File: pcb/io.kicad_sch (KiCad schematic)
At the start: 31 parts, among them Q3 2N7002, Q4 2N7002, Q5 2N7002, Q6 2N7002, Q7 BT148, Q8 BT148

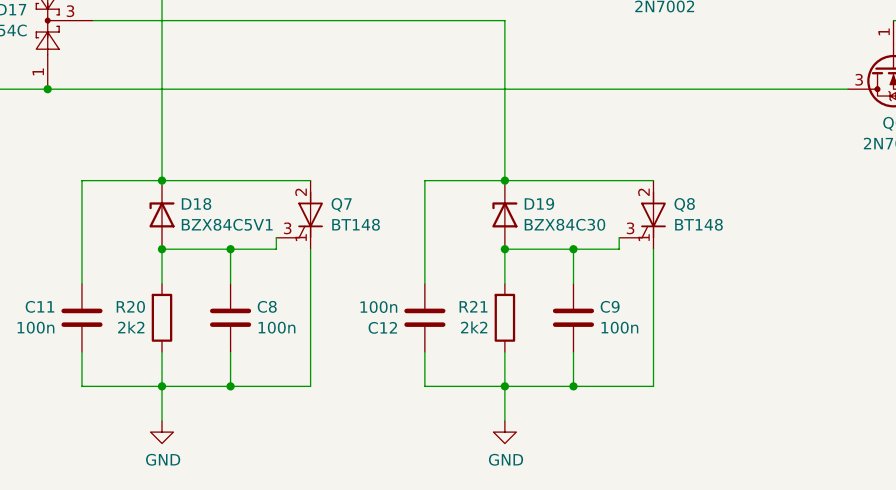
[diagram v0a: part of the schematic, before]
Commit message: Add protection on internal inputs, divide stepdown voltage measuring by 2.
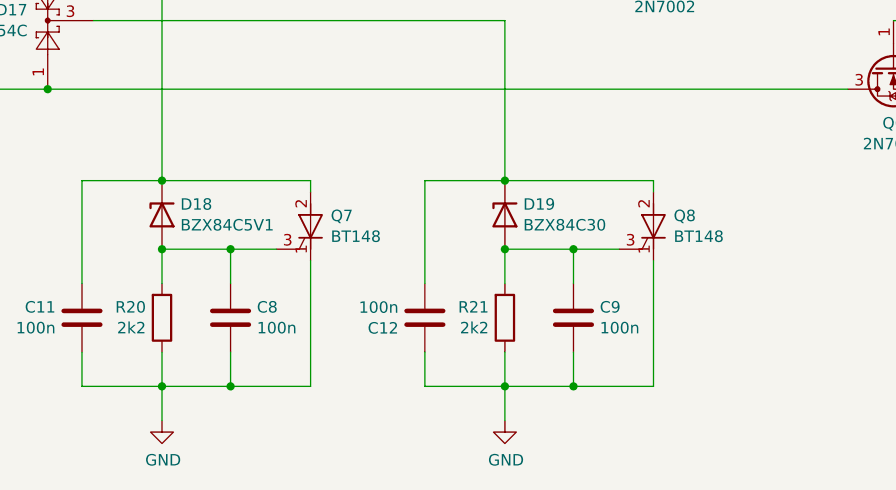
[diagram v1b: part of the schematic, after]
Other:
- moved on the sheet: Q7, Q8
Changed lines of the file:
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@@
+    (stroke (width 0) (type default))
+  )
+  (wire (pts (xy 158.75 160.02) (xy 142.24 160.02))
     (stroke (width 0) (type default))
   )
@@
     (stroke (width 0) (type default))
   )
-  (wire (pts (xy 158.75 167.64) (xy 158.75 182.88))
+  (wire (pts (xy 158.75 161.29) (xy 158.75 160.02))
+    (stroke (width 0) (type default))
+  )
+  (wire (pts (xy 158.75 168.91) (xy 158.75 182.88))
     (stroke (width 0) (type default))
   )
@@
     (stroke (width 0) (type default))
   )
-  (wire (pts (xy 142.24 160.02) (xy 158.75 160.02))
-    (stroke (width 0) (type default))
-  )
   (wire (pts (xy 142.24 186.69) (xy 142.24 182.88))
     (stroke (width 0) (type default))
@@
     (stroke (width 0) (type default))
   )
-  (wire (pts (xy 104.14 160.02) (xy 120.65 160.02))
-    (stroke (width 0) (type default))
-  )
-  (wire (pts (xy 116.84 167.64) (xy 116.84 166.37))
-    (stroke (width 0) (type default))
-  )
   (wire (pts (xy 185.42 142.24) (xy 194.31 142.24))
     (stroke (width 0) (type default))
@@
     (stroke (width 0) (type default))
   )
+  (wire (pts (xy 120.65 160.02) (xy 104.14 160.02))
+    (stroke (width 0) (type default))
+  )
   (wire (pts (xy 59.69 36.83) (xy 66.04 36.83))
     (stroke (width 0) (type default))
@@
     (stroke (width 0) (type default))
   )
-  (wire (pts (xy 120.65 167.64) (xy 120.65 182.88))
+  (wire (pts (xy 120.65 168.91) (xy 120.65 182.88))
     (stroke (width 0) (type default))
   )
@@
     (stroke (width 0) (type default))
   )
-  (wire (pts (xy 154.94 167.64) (xy 154.94 166.37))
-    (stroke (width 0) (type default))
-  )
   (wire (pts (xy 129.54 91.44) (xy 129.54 111.76))
     (stroke (width 0) (type default))
@@
   )
   (wire (pts (xy 142.24 167.64) (xy 149.86 167.64))
+    (stroke (width 0) (type default))
+  )
+  (wire (pts (xy 120.65 161.29) (xy 120.65 160.02))
     (stroke (width 0) (type default))
   )
@@
     )
   )
-  (symbol (lib_id "Device:Q_SCR_KAG") (at 120.65 163.83 0) (unit 1)
-    (in_bom yes) (on_board yes) (dnp no)
-    (property "Reference" "Q7" (at 122.8852 162.6616 0)
-      (effects (font (size 1.27 1.27)) (justify left))
-    )
-    (property "Value" "BT148" (at 122.8852 164.973 0)
-      (effects (font (size 1.27 1.27)) (justify left))
-    )
-    (property "Footprint" "Package_TO_SOT_SMD:SOT-223" (at 120.65 163.83 90)
-      (effects (font (size 1.27 1.27)) hide)
-    )
-    (property "Datasheet" "~" (at 120.65 163.83 90)
-      (effects (font (size 1.27 1.27)) hide)
-    )
-    (property "LCSC" "C256433" (at 120.65 163.83 0)
+  (symbol (lib_id "Device:Q_SCR_KAG") (at 120.65 165.1 0) (unit 1)
+    (in_bom yes) (on_board yes) (dnp no)
+    (property "Reference" "Q7" (at 122.8852 163.9316 0)
+      (effects (font (size 1.27 1.27)) (justify left))
+    )
+    (property "Value" "BT148" (at 122.8852 166.243 0)
+      (effects (font (size 1.27 1.27)) (justify left))
+    )
+    (property "Footprint" "Package_TO_SOT_SMD:SOT-223" (at 120.65 165.1 90)
+      (effects (font (size 1.27 1.27)) hide)
+    )
+    (property "Datasheet" "~" (at 120.65 165.1 90)
+      (effects (font (size 1.27 1.27)) hide)
+    )
+    (property "LCSC" "C256433" (at 120.65 165.1 0)
       (effects (font (size 1.27 1.27)) hide)
     )
@@
     )
   )
-  (symbol (lib_id "Device:Q_SCR_KAG") (at 158.75 163.83 0) (unit 1)
-    (in_bom yes) (on_board yes) (dnp no)
-    (property "Reference" "Q8" (at 160.9852 162.6616 0)
-      (effects (font (size 1.27 1.27)) (justify left))
-    )
-    (property "Value" "BT148" (at 160.9852 164.973 0)
-      (effects (font (size 1.27 1.27)) (justify left))
-    )
-    (property "Footprint" "Package_TO_SOT_SMD:SOT-223" (at 158.75 163.83 90)
-      (effects (font (size 1.27 1.27)) hide)
-    )
-    (property "Datasheet" "~" (at 158.75 163.83 90)
-      (effects (font (size 1.27 1.27)) hide)
-    )
-    (property "LCSC" "C256433" (at 158.75 163.83 0)
-      (effects (font (size 1.27 1.27)) hide)
-    )
+  (symbol (lib_id "Device:Q_SCR_KAG") (at 158.75 165.1 0) (unit 1)
+    (in_bom yes) (on_board yes) (dnp no)
+    (property "Reference" "Q8" (at 160.9852 163.9316 0)
+      (effects (font (size 1.27 1.27)) (justify left))
+    )
+    (property "Value" "BT148" (at 160.9852 166.243 0)
+      (effects (font (size 1.27 1.27)) (justify left))
+    )
+    (property "Footprint" "Package_TO_SOT_SMD:SOT-223" (at 158.75 165.1 90)
+      (effects (font (size 1.27 1.27)) hide)
+    )
+    (property "Datasheet" "~" (at 158.75 165.1 90)
+      (effects (font (size 1.27 1.27)) hide)
+    )
+    (property "LCSC" "C256433" (at 158.75 165.1 0)
+      (effects (font (size 1.27 1.27)) hide)
+    )
